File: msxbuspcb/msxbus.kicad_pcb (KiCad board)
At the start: 2 copper layers, 9 parts, among them J1 RPi_GPIO, P1 CONN_02X25, P2 CONN_02X25, P4 CONN_01X03, U1 EMP240

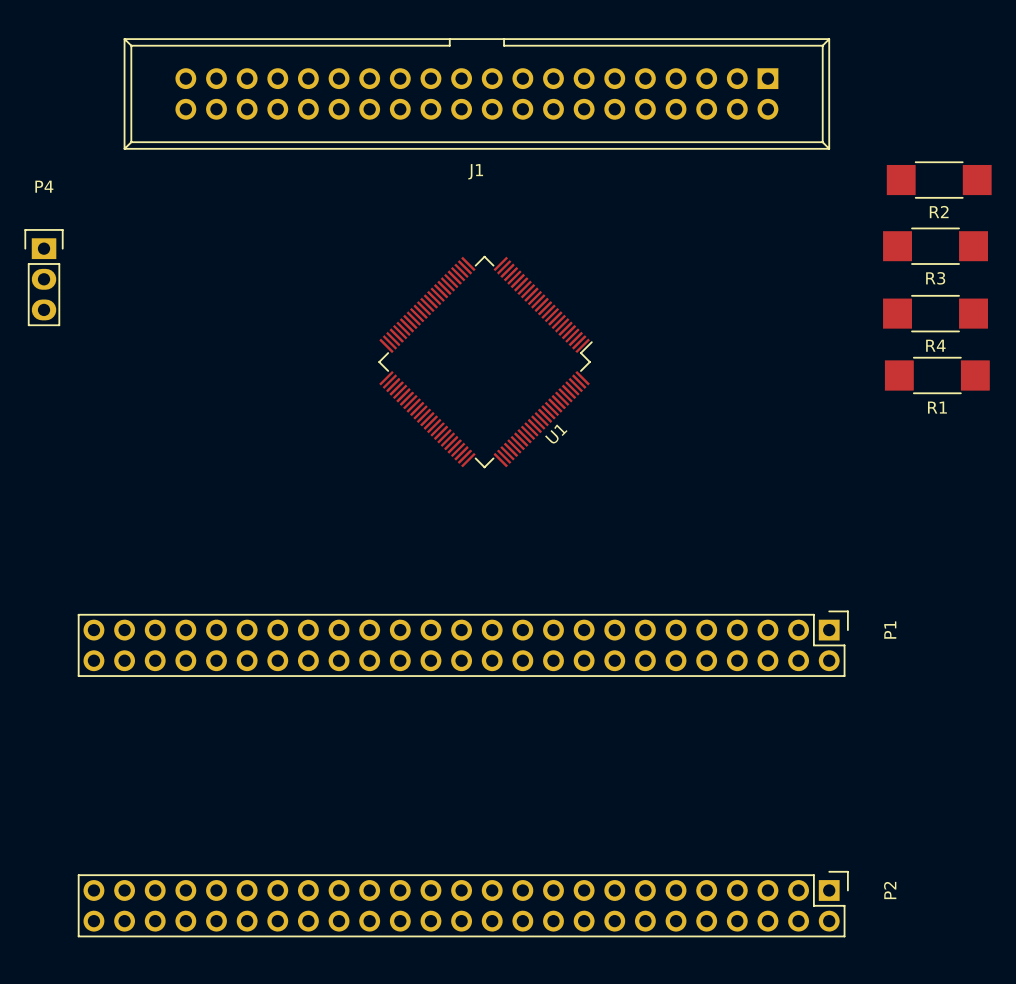
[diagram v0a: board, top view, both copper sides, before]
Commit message: route for pcb
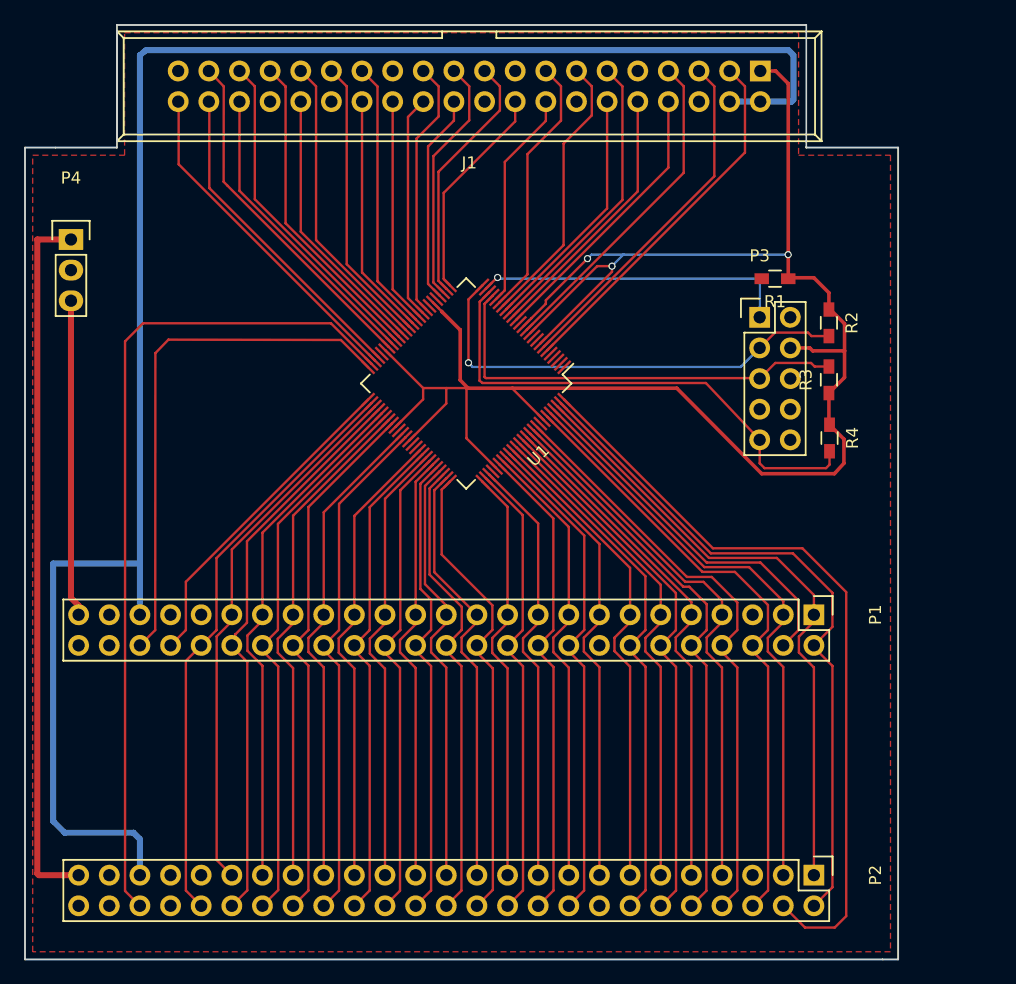
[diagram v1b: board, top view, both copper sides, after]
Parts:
- added P3: CONN_02X05, Pin_Headers:Pin_Header_Straight_2x05, F.Cu at (167.6, 100.4)
- R1, R2, R3, R4: footprint Resistors_SMD:R_2010_HandSoldering -> Resistors_SMD:R_0603_HandSoldering
- moved R1 15.7 mm to (168.9, 97.2)
- moved R2 15.0 mm to (173.3, 100.9), turned to 270 degrees
- moved R3 14.2 mm to (173.3, 105.6), turned to 90 degrees
- moved R4 13.5 mm to (173.4, 110.4), turned to 270 degrees
- moved P4 2.36 mm to (110.5, 94.0)
- moved U1 2.34 mm to (143.3, 105.9)
- moved P2 1.80 mm to (172.1, 146.7)
- moved P1 1.80 mm to (172.1, 125.1)
- moved J1 0.90 mm to (167.6, 80.0)
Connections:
- net /3V3 renamed +3V3
- net /CLK3 renamed Net-(U1-Pad64)
- J1 pad 15: /SLTSL1 -> /MSLTSL1
- U1 pad 100: /SLTSL0 -> /SLTSL1
- U1 pad 30: /MD11 -> Net-(U1-Pad30)
- U1 pad 33: /MD08 -> /MD11
- U1 pad 34: /MD11 -> /MD08
- U1 pad 49: Net-(U1-Pad49) -> /SW2
- U1 pad 50: Net-(U1-Pad50) -> /SW1
- U1 pad 51: /SW2 -> /SWOUT
- U1 pad 52: /SW1 -> /CLOCK
- U1 pad 53: /SWOUT -> /D7
- U1 pad 54: /D7 -> /D6
- U1 pad 55: /D6 -> /D5
- U1 pad 56: /D5 -> /D4
- U1 pad 57: /D4 -> /D3
- U1 pad 58: /D3 -> /D2
- U1 pad 61: /D2 -> /D1
- U1 pad 62: /CLOCK -> /D0
- U1 pad 66: /D1 -> /A5
- U1 pad 67: /D0 -> /A4
- U1 pad 68: /A5 -> /A3
- U1 pad 97: /CS1 -> /SLTSL0
- U1 pad 98: /CS2 -> /CS1
- U1 pad 99: /SLTSL1 -> /CS2
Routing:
- net +3V3: track 0.00 -> 159.3 mm, vias 0 -> 3
- net +5V: track 0.00 -> 149.4 mm
- net /SW2: track 0.00 -> 69.8 mm
- net /SLTSL1: track 0.00 -> 63.2 mm
- net Net-(P2-Pad49): track 0.00 -> 58.9 mm
- net /CS2: track 0.00 -> 56.9 mm
- net /CS1: track 0.00 -> 52.0 mm
- net /RFSH: track 0.00 -> 51.3 mm
- net /CS12: track 0.00 -> 49.5 mm
- net /INT: track 0.00 -> 49.4 mm
- net /CLOCK: track 0.00 -> 48.6 mm
- net /D6: track 0.00 -> 47.2 mm
- net /BUSDIR: track 0.00 -> 47.1 mm
- net /D4: track 0.00 -> 45.8 mm
- net /MERQ: track 0.00 -> 45.4 mm
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- added copper zone on F.Cu, net /GND
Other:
- board outline added: 72.4 x 77.5 mm
- net class 3V3 added: clearance 0.18, trace_width 0.2, via_dia 0.6, via_drill 0.4
- net class 5V added: clearance 0.18, trace_width 0.5, via_dia 0.6, via_drill 0.4
- net class Default: clearance 0.2 -> 0.18; trace_width 0.25 -> 0.2
- rule trace_clearance: 0.2 -> 0.18
